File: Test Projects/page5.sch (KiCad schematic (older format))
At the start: 23 parts, among them P21 CONN_01X05, P89 CONN_01X04, U13 SF-4052, U14 SF-4052, U15 SF-4052, U16 SF-4052, U17 SF-4052, U18 SF-4052, U19 SF-4052, U20 SF-4052, U21 SF-4052, U22 SF-4052

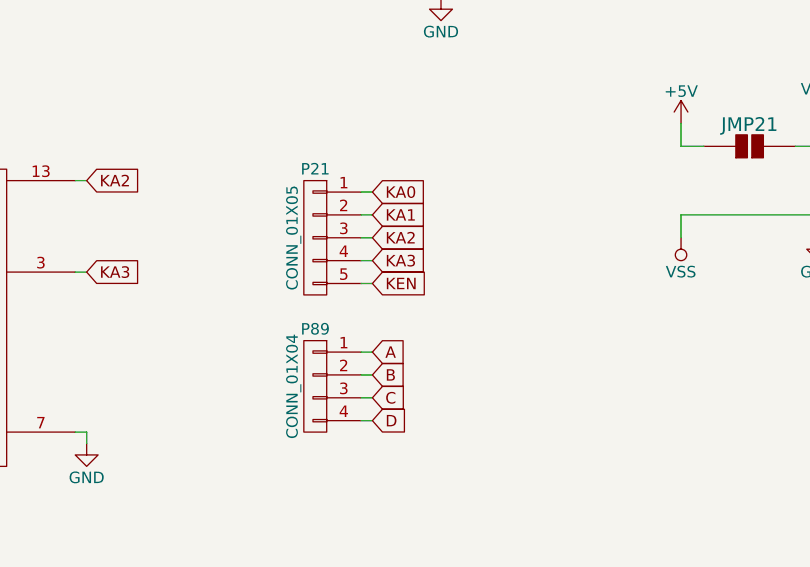
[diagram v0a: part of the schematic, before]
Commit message: layout
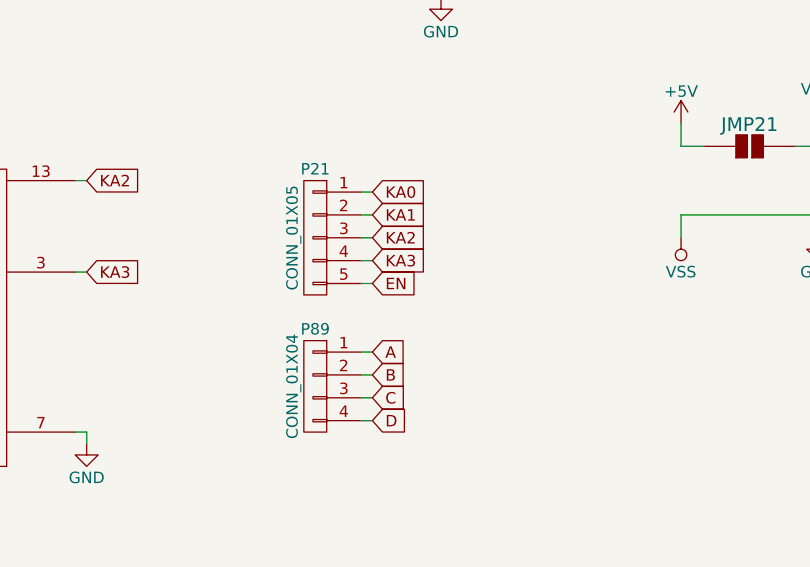
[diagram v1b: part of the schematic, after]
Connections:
- net KEN is gone; now on net EN: P21.5 (P5)
